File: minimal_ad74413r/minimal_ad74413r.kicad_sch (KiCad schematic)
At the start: 50 parts, among them J1 CLP-102-02-G-D-BE, J2 CLP-102-02-G-D-BE, J3 CLP-102-02-G-D-BE, J4 CLP-102-02-G-D-BE, J5 CLP-102-02-G-D-BE, J6 CLP-102-02-G-D-BE, J7 CLP-114-02-G-D-BE, U1 AD74413RBCPZ

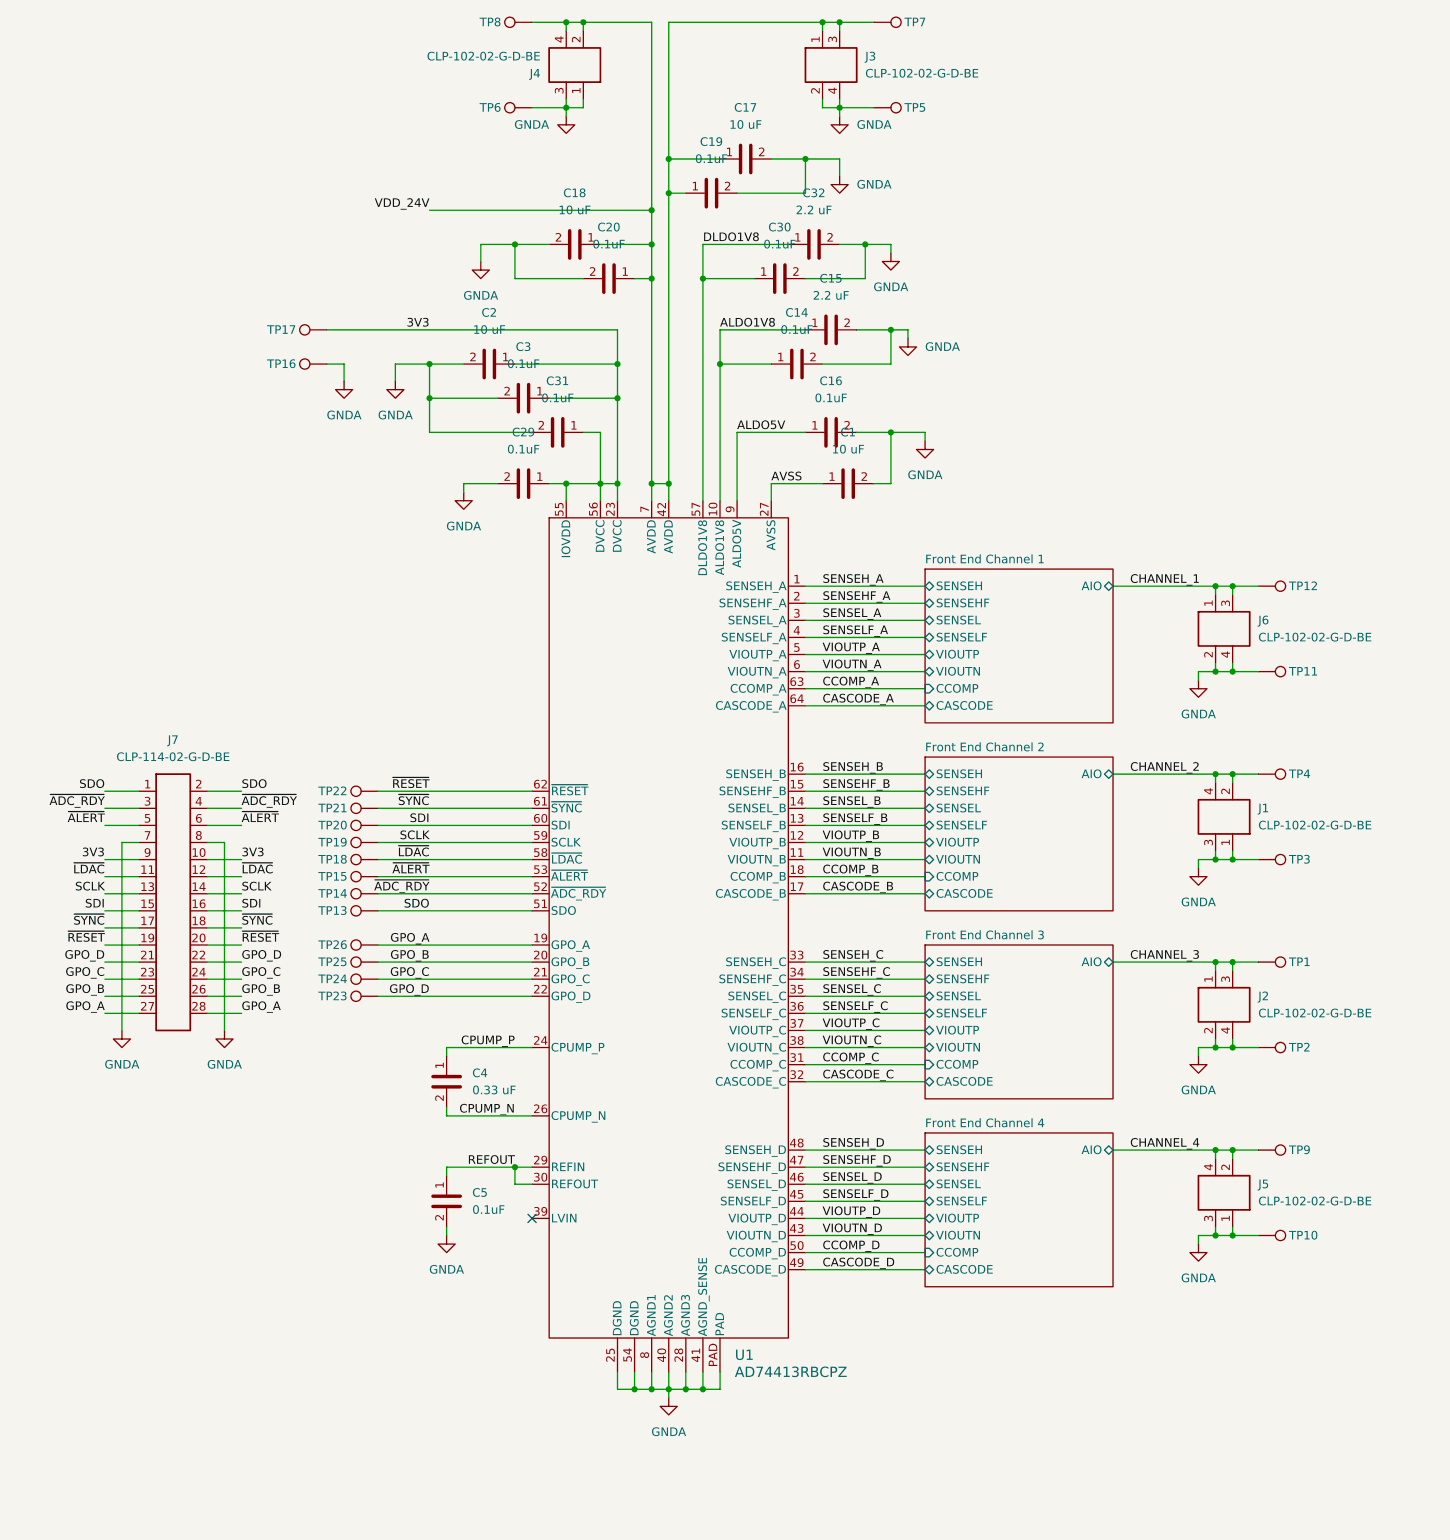
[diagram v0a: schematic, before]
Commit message: Minor updates
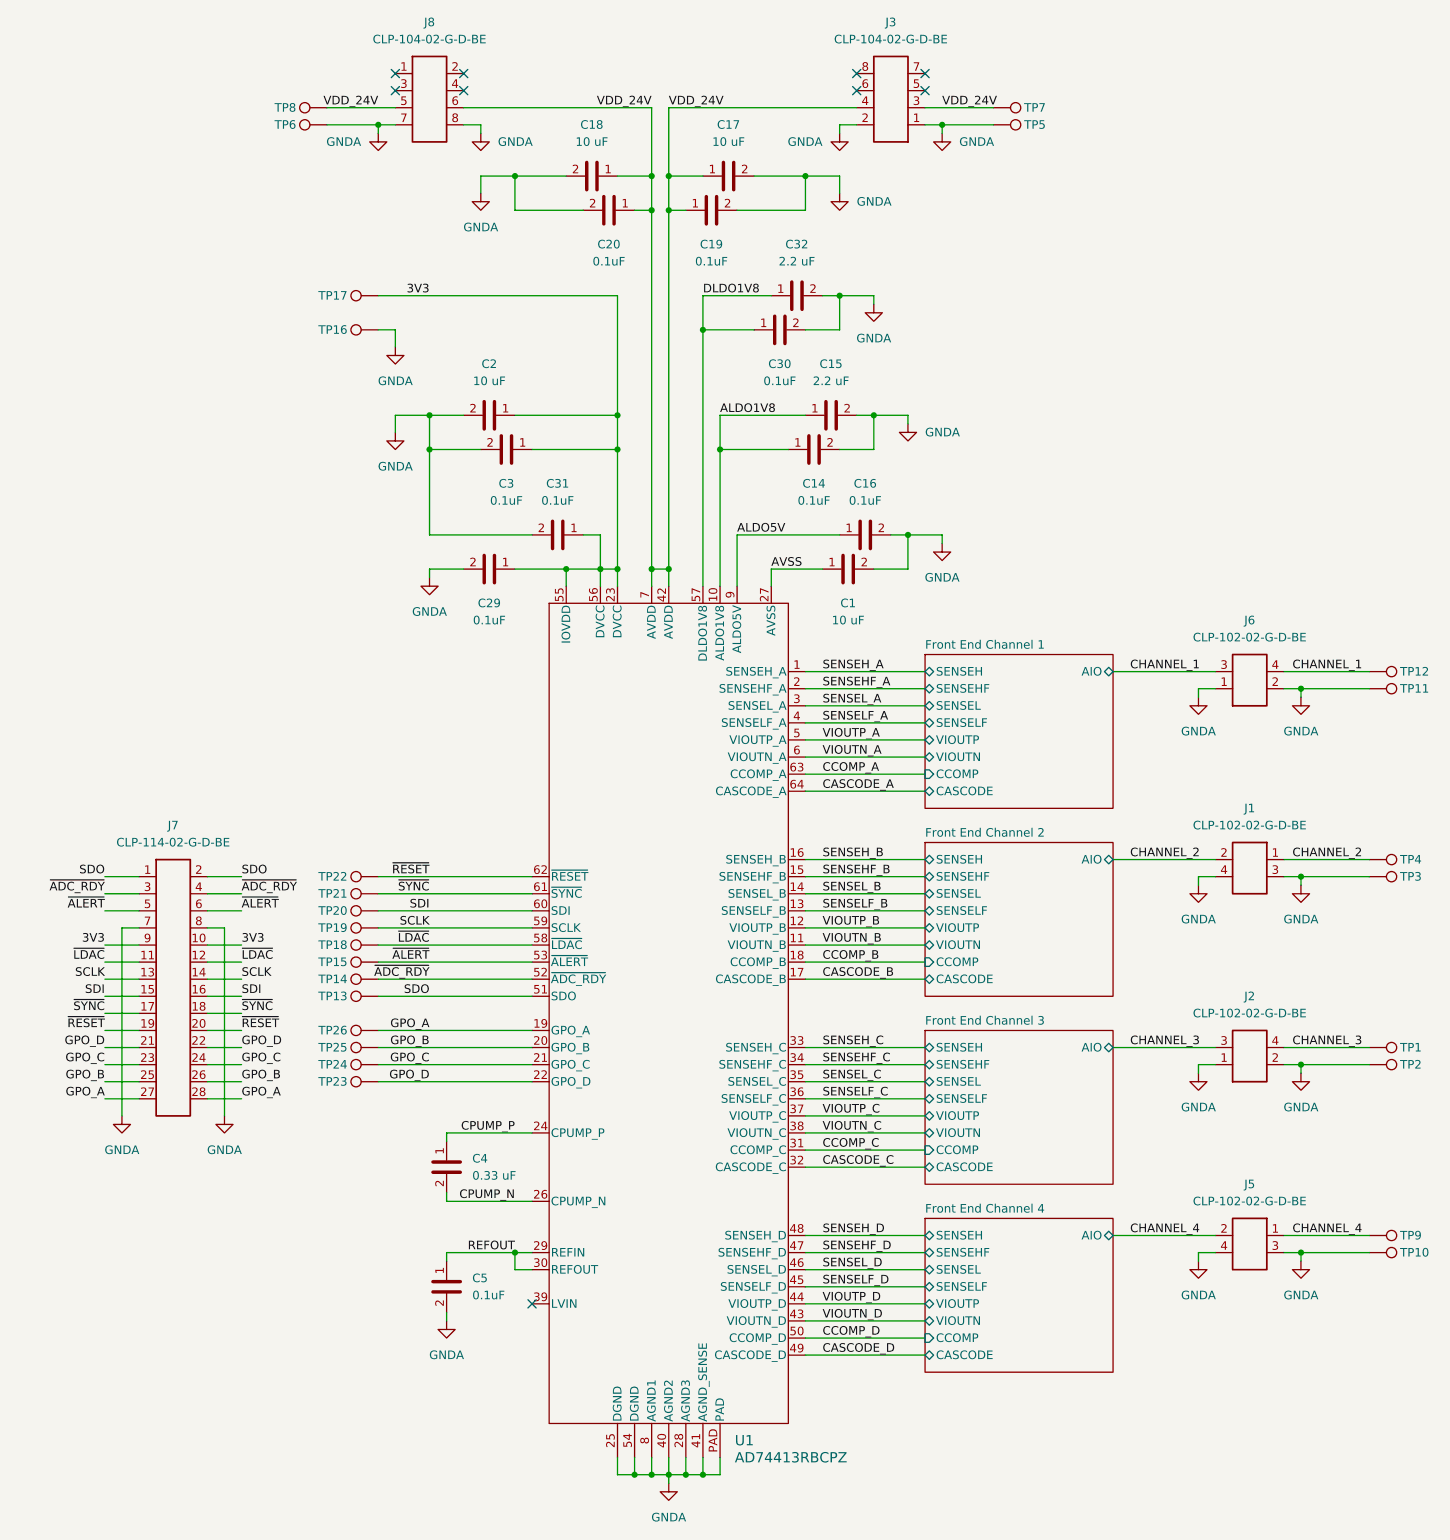
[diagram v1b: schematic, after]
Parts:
- removed J3, J4: CLP-102-02-G-D-BE, connector_footprints:CLP-102-02-G-D-BE, symbol UNITED_CONNECTORS_DATA_BASE:J_CLP-102-02-G-D-BE
- added J3, J8: CLP-104-02-G-D-BE, connector_footprints:CLP-104-02-G-D-BE, symbol UNITED_CONNECTORS_DATA_BASE:J_CLP-104-02-G-D-BE
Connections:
- net CHANNEL_1: now also J6.4; no longer J6.1
- net CHANNEL_2: now also J1.1; no longer J1.4
- net CHANNEL_3: now also J2.4; no longer J2.1
- net CHANNEL_4: now also J5.1; no longer J5.4
- net GNDA: now also J1.4, J2.1, J5.4, J6.1, J3.1, J3.2, J8.7, J8.8; no longer J1.1, J2.4, J5.1, J6.4
- net VDD_24V: now also J3.3, J3.4, J8.5, J8.6
- no-connect marks 1 -> 9
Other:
- moved on the sheet: C1, C14, C15, C16, C17, C18, C19, C2, C20, C29, C3, C30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
